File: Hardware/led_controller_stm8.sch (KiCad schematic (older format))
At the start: 11 parts, among them J1 WS_LED, J2 PROGRAMMING, J3 EXT_BTN, SW1 SW_Push, U1 STM8S103F3

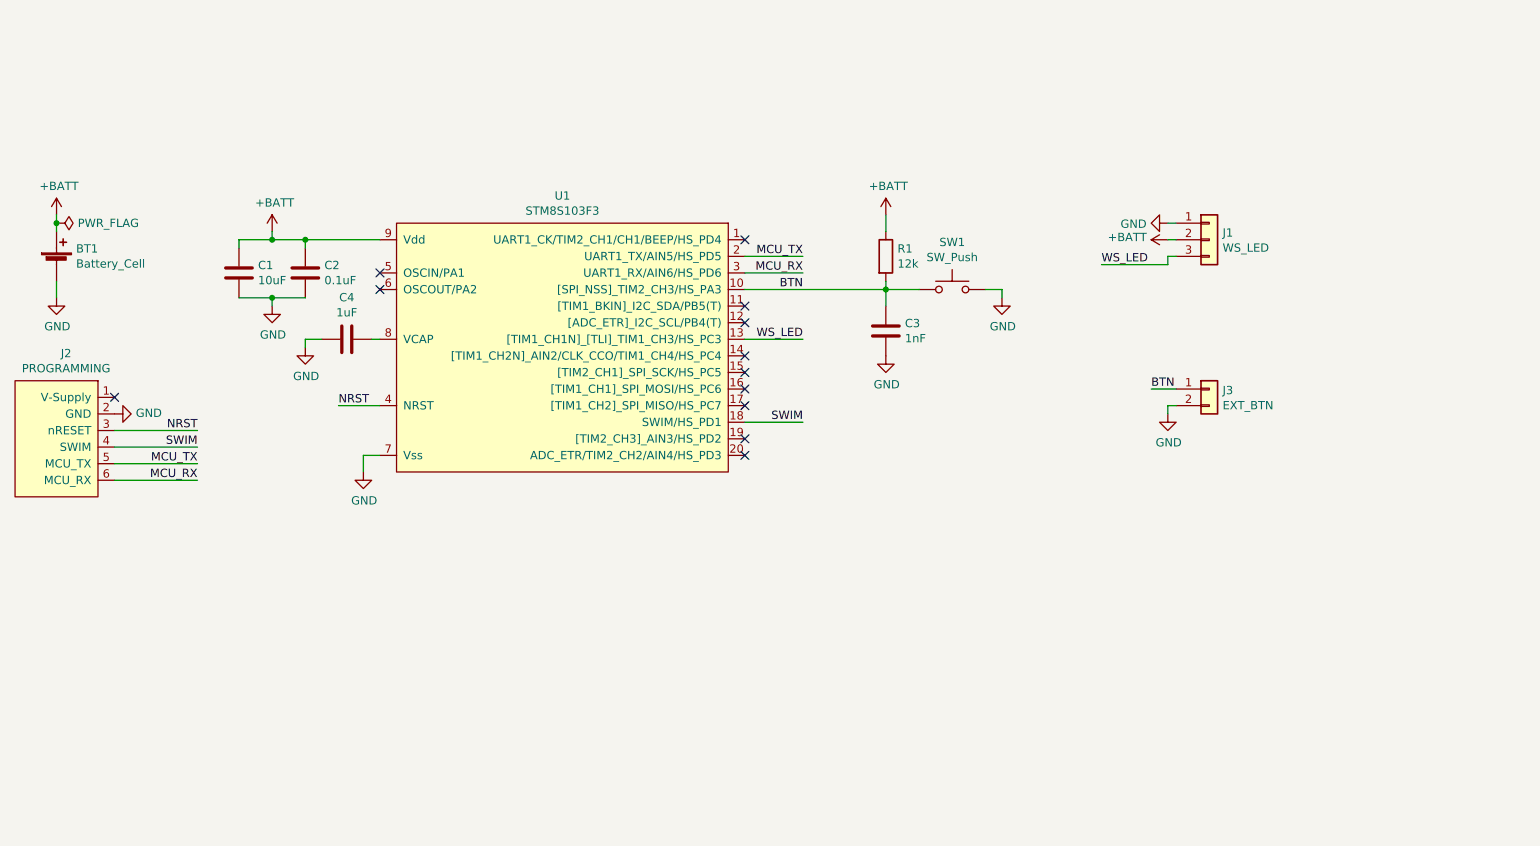
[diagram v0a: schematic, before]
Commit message: add pcb
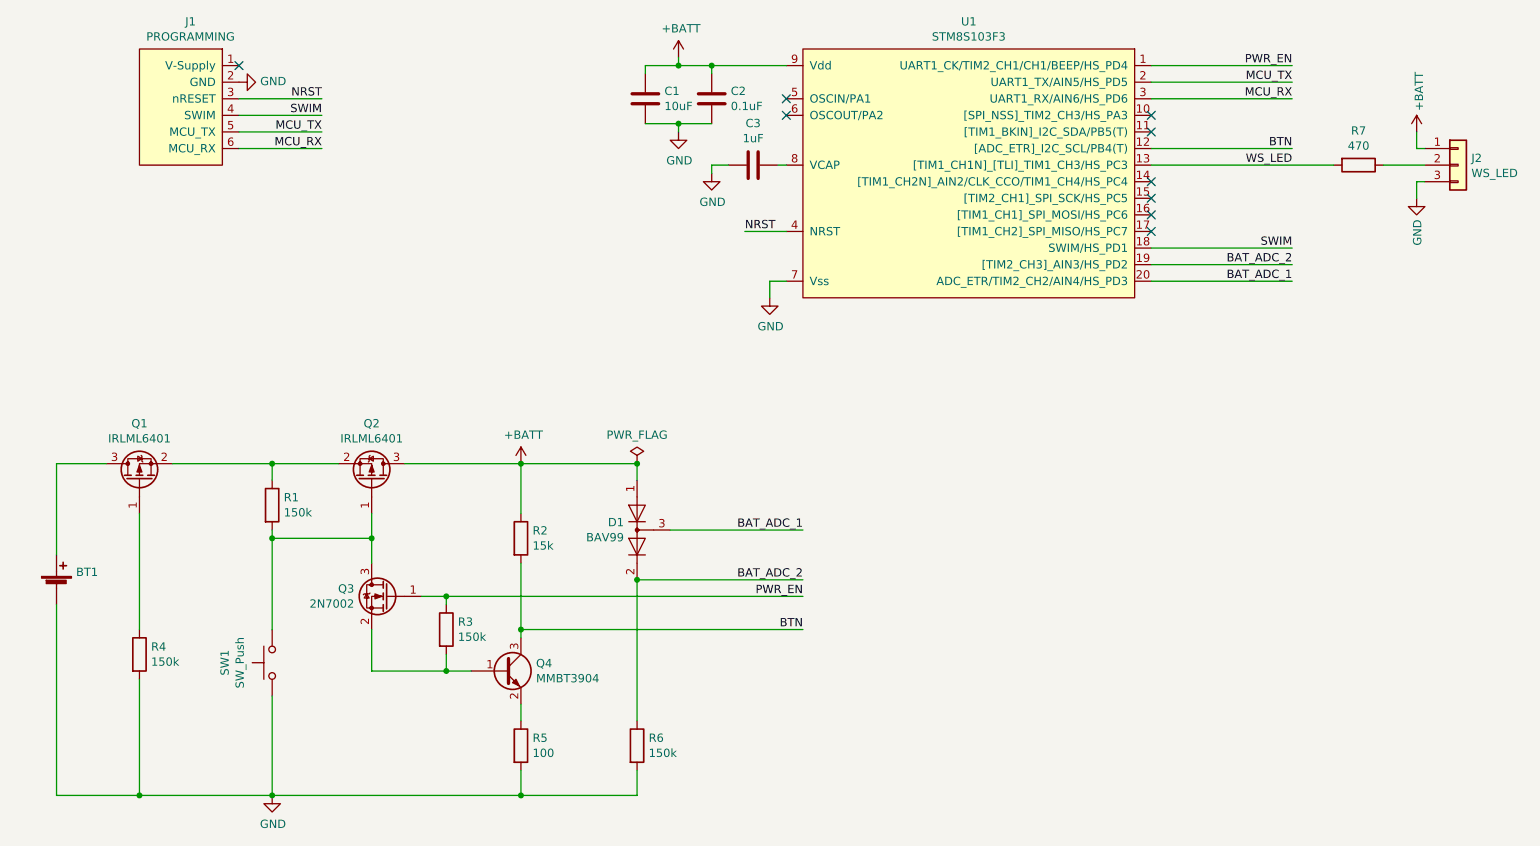
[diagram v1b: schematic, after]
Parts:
- removed C3: 1nF, Capacitor_SMD:C_0805_2012Metric_Pad1.15x1.40mm_HandSolder, symbol Device:C
- removed J3: EXT_BTN, Connector_JST:JST_PH_B2B-PH-K_1x02_P2.00mm_Vertical, symbol Connector_Generic:Conn_01x02
- added D1: BAV99, Package_TO_SOT_SMD:SOT-23, symbol Diode:BAV99
- added Q1, Q2: IRLML6401, Package_TO_SOT_SMD:SOT-23, symbol Transistor_FET:IRLML6401
- added Q3: 2N7002, Package_TO_SOT_SMD:SOT-23, symbol Transistor_FET:2N7002
- added Q4: MMBT3904, Package_TO_SOT_SMD:SOT-23, symbol Transistor_BJT:MMBT3904
- added R2: 15k, Resistor_SMD:R_0805_2012Metric_Pad1.15x1.40mm_HandSolder, symbol Device:R
- added R3, R4, R6: 150k, Resistor_SMD:R_0805_2012Metric_Pad1.15x1.40mm_HandSolder, symbol Device:R
- added R5: 100, Resistor_SMD:R_0805_2012Metric_Pad1.15x1.40mm_HandSolder, symbol Device:R
- added R7: 470, Resistor_SMD:R_0805_2012Metric_Pad1.15x1.40mm_HandSolder, symbol Device:R
- J2: renamed from J1; footprint Connector_JST:JST_PH_B3B-PH-K_1x03_P2.00mm_Vertical -> Connector_JST:JST_XH_B3B-XH-A_1x03_P2.50mm_Vertical
- R1: value 12k -> 150k
- renumbered C4 to C3, J2 to J1
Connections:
- net +BATT: now also J2.1 (Pin_1), D1.1 (K), Q2.3 (D), R2.1; no longer BT1.1 (+), J2.2 (Pin_2), R1.1
- net BTN: now also U1.12 ([ADC_ETR]_I2C_SCL/PB4(T)), Q4.3 (C), R2.2; no longer R1.2, SW1.1, U1.10 ([SPI_NSS]_TIM2_CH3/HS_PA3)
- net GND: now also J2.3 (Pin_3), SW1.1, R4.2, R5.2, R6.2; no longer J2.1 (Pin_1), SW1.2
- net WS_LED: now also R7.2; no longer J2.3 (Pin_3)
- net PWR_EN: now reaches U1.1 (UART1_CK/TIM2_CH1/CH1/BEEP/HS_PD4)
- net PWR_EN: now also Q3.1 (G), R3.1
- net BAT_ADC_2: now reaches U1.19 ([TIM2_CH3]_AIN3/HS_PD2)
- net BAT_ADC_2: now also D1.2 (A), R6.1
- net BAT_ADC_1: now reaches U1.20 (ADC_ETR/TIM2_CH2/AIN4/HS_PD3)
- net BAT_ADC_1: now also D1.3 (K)
- new net: J2.2 (Pin_2), R7.1
- new net: BT1.1 (+), Q1.3 (D)
- new net: Q1.1 (G), R4.1
- new net: Q1.2 (S), Q2.2 (S), R1.1
- new net: Q2.1 (G), Q3.3 (D), R1.2, SW1.2
- new net: Q3.2 (S), Q4.1 (B), R3.2
- new net: Q4.2 (E), R5.1
- no-connect marks 12 -> 9
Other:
- moved on the sheet: BT1, C1, C2, C3, J1, J2, U1
